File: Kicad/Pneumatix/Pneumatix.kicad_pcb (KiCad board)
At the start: 2 copper layers, 33.1 x 59.4 mm, 16 parts, among them J1 436500404, J2 142-0701-801, J3 Conn_01x04_Socket, U1 E22-400T33S

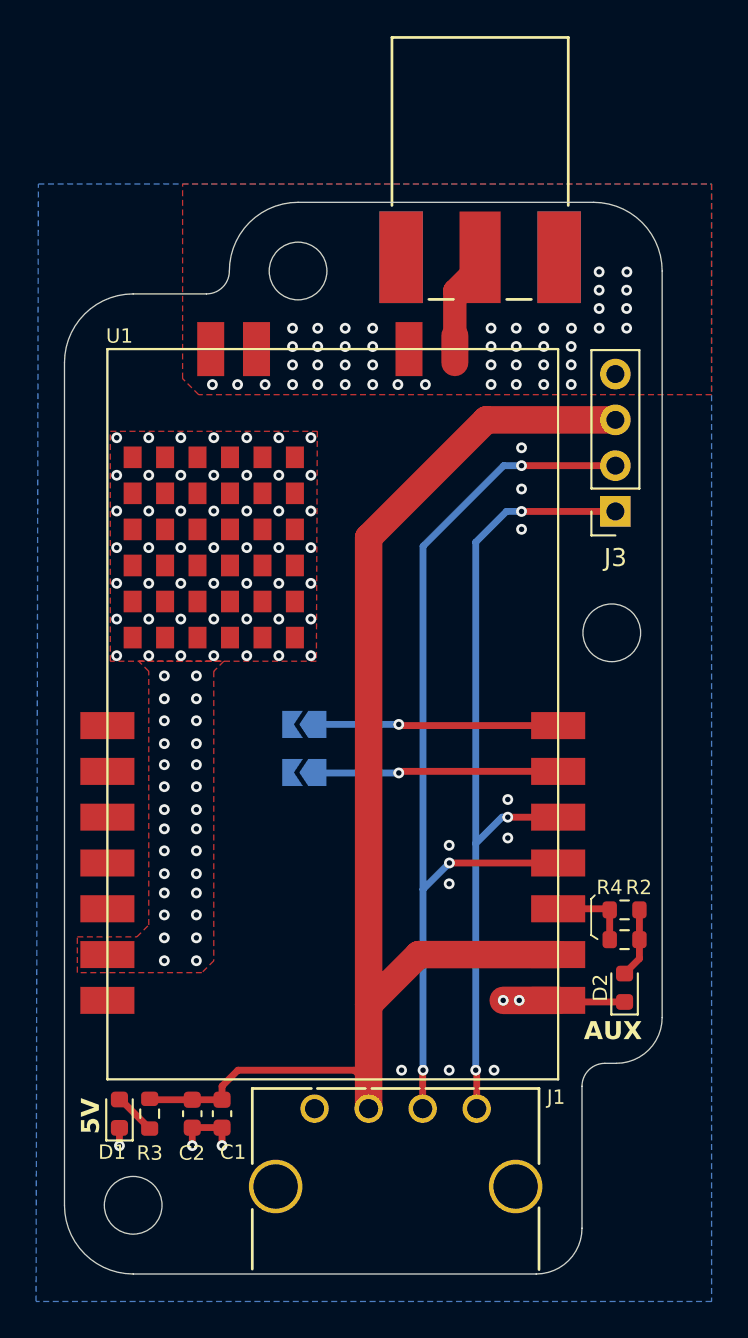
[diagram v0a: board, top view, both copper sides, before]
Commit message: wip: add pu/pd for M0 and M1, remake traces and swap gnd/signal/passive components plane
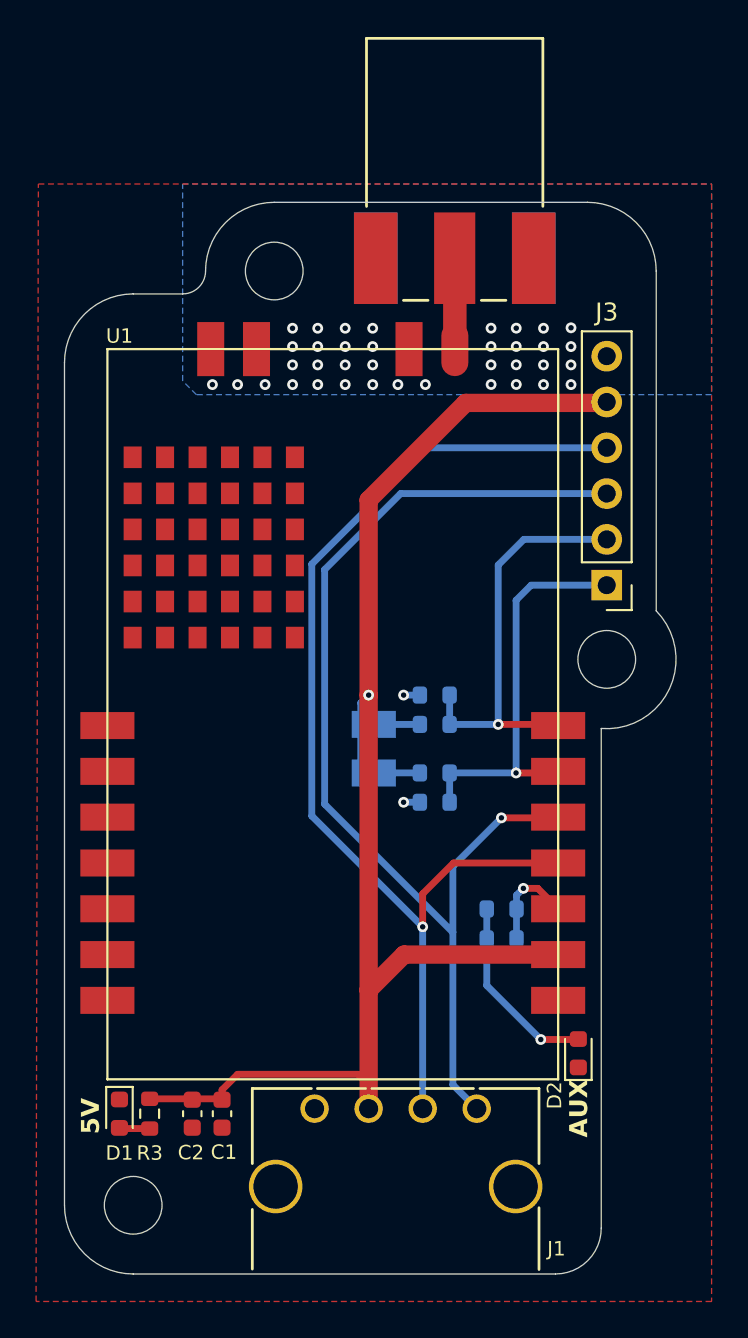
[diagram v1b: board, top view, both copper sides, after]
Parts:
- added R5: 1.5k, Resistor_SMD:R_0603_1608Metric, B.Cu at (20.5, 31.6)
- added R6: 1.5k, Resistor_SMD:R_0603_1608Metric, B.Cu at (20.5, 33.3)
- added R7: 1.5k, Resistor_SMD:R_0603_1608Metric, B.Cu at (20.5, 29.0)
- added R8: 1.5k, Resistor_SMD:R_0603_1608Metric, B.Cu at (20.5, 27.3)
- J3: value Conn_01x04_Socket -> Conn_01x06_Socket; footprint Connector_PinSocket_2.54mm:PinSocket_1x04_P2.54mm_Vertical -> Connector_PinHeader_2.54mm:PinHeader_1x06_P2.54mm_Vertical
- R2, R4: moved to B.Cu
- moved R2 6.82 mm to (24.2, 39.2), turned to 180 degrees
- moved R4 6.82 mm to (24.2, 40.8), turned to 180 degrees
- moved JP1 4.71 mm to (17.2, 31.6)
- moved JP2 4.69 mm to (17.2, 29.0)
- moved D2 4.45 mm to (28.5, 47.2)
- moved J3 4.12 mm to (30.1, 21.2)
- moved H3 1.50 mm to (30.1, 25.3)
- moved J2 1.41 mm to (21.6, 3.10)
- moved H1 1.32 mm to (11.6, 3.81)
- turned D1 to -90 degrees
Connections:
- J3 pad 1: LORA_TX -> LORA_M1
- J3 pad 2: LORA_RX -> LORA_M0
- J3 pad 3: +5V -> LORA_TX
- J3 pad 4: GND -> LORA_RX
- JP1 pad 2: GND -> +5V
- JP2 pad 2: GND -> +5V
- U1 pad 6: Net-(JP2-A) -> LORA_M1
- U1 pad 7: Net-(JP1-A) -> LORA_M0
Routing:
- net LORA_M0: track 0.00 -> 23.0 mm, vias 0 -> 1
- net LORA_M1: track 0.00 -> 22.5 mm, vias 0 -> 1
- net LORA_TX: track 45.1 -> 61.4 mm, vias 3 -> 1
- net Net-(JP2-A): track 13.5 -> 1.83 mm, vias 1 -> 0
- net Net-(JP1-A): track 13.5 -> 1.83 mm, vias 1 -> 0
- net LORA_RX: track 51.8 -> 61.8 mm, vias 3 -> 1
- net GND: track 11.5 -> 1.80 mm, vias 137 -> 39
- net Net-(D2-A): track 3.87 -> 10.5 mm, vias 0 -> 1
- net +5V: track 74.7 -> 79.1 mm, vias 0 -> 1
- net Net-(U1-ANT): track 5.86 -> 5.03 mm
- net Net-(U1-AUX): track 4.53 -> 5.35 mm, vias 0 -> 1
- net Net-(D1-A): track 2.34 -> 1.64 mm
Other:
- board size 33.1 x 59.4 mm -> 33.9 x 59.4 mm
